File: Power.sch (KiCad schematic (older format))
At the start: 23 parts, among them U13 L78L12_SOT89, U14 MP4462, U3 L78L12_SOT89, U4 LP2985-3.3

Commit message: Lots of routing done
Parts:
- added C73: 1uF, Capacitor_SMD:C_0402_1005Metric, symbol Device:C_Small
- added C77: 10nF, Capacitor_SMD:C_0402_1005Metric, symbol Device:C_Small
- added C78: 2.2uF, Capacitor_SMD:C_0603_1608Metric, symbol Device:C_Small
- added U16: LP2985-3.3, Package_TO_SOT_SMD:SOT-23-5, symbol Regulator_Linear:LP2985-3.3
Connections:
- net labels added: +3V3_1, +3V3_2
- net labels removed: +3V3
- wire segments 51 -> 64
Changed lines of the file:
@@
 Connection ~ 8600 3600
-$Comp
-L power:+3V3 #PWR0123
-U 1 1 603A9DDE
-P 8600 3500
-F 0 "#PWR0123" H 8600 3350 50  0001 C CNN
-F 1 "+3V3" H 8615 3673 50  0000 C CNN
-F 2 "" H 8600 3500 50  0001 C CNN
-F 3 "" H 8600 3500 50  0001 C CNN
-	1    8600 3500
-	1    0    0    -1
-$EndComp
-Connection ~ 8600 3500
 $Comp
 L Device:C_Small C?
@@
 	7150 3050 7150 4050
 Wire Notes Line
-	7150 4050 8900 4050
-Wire Notes Line
-	8900 4050 8900 3050
-Wire Notes Line
-	8900 3050 7150 3050
+	10650 4050 10650 3050
 Text Notes 7200 3200 0    79   ~ 16
 3V3 LDO Regulator
@@
 	7050 4850 7050 4750
 Connection ~ 7050 4750
+$Comp
+L Regulator_Linear:LP2985-3.3 U16
+U 1 1 61219C4E
+P 9550 3600
+F 0 "U16" H 9550 3942 50  0000 C CNN
+F 1 "LP2985-3.3" H 9550 3851 50  0000 C CNN
+F 2 "Package_TO_SOT_SMD:SOT-23-5" H 9550 3925 50  0001 C CNN
+F 3 "http://www.ti.com/lit/ds/symlink/lp2985.pdf" H 9550 3600 50  0001 C CNN
+	1    9550 3600
+	1    0    0    -1
+$EndComp
+$Comp
+L Device:C_Small C?
+U 1 1 61219C54
+P 9050 3800
+AR Path="/61219C54" Ref="C?"  Part="1"
+AR Path="/60308500/61219C54" Ref="C73"  Part="1"
+F 0 "C73" H 9142 3846 50  0000 L CNN
+F 1 "1uF" H 9100 3800 50  0000 L CNN
+F 2 "Capacitor_SMD:C_0402_1005Metric" H 9050 3800 50  0001 C CNN
+F 3 "~" H 9050 3800 50  0001 C CNN
+	1    9050 3800
+	1    0    0    -1
+$EndComp
+$Comp
+L Device:C_Small C?
+U 1 1 61219C5A
+P 10050 3800
+AR Path="/61219C5A" Ref="C?"  Part="1"
+AR Path="/60308500/61219C5A" Ref="C77"  Part="1"
+F 0 "C77" H 10142 3846 50  0000 L CNN
+F 1 "10nF" H 10100 3800 50  0000 L CNN
+F 2 "Capacitor_SMD:C_0402_1005Metric" H 10050 3800 50  0001 C CNN
+F 3 "~" H 10050 3800 50  0001 C CNN
+	1    10050 3800
+	1    0    0    -1
+$EndComp
+Wire Wire Line
+	10050 3700 10050 3600
+Wire Wire Line
+	10050 3600 9950 3600
+Wire Wire Line
+	9050 3700 9050 3600
+Wire Wire Line
+	9050 3600 9150 3600
+Connection ~ 9050 3600
+Wire Wire Line
+	9050 3500 9150 3500
+$Comp
+L Device:C_Small C?
+U 1 1 61219C66
+P 10350 3800
+AR Path="/61219C66" Ref="C?"  Part="1"
+AR Path="/60308500/61219C66" Ref="C78"  Part="1"
+F 0 "C78" H 10442 3846 50  0000 L CNN
+F 1 "2.2uF" H 10400 3800 50  0000 L CNN
+F 2 "Capacitor_SMD:C_0603_1608Metric" H 10350 3800 50  0001 C CNN
+F 3 "~" H 10350 3800 50  0001 C CNN
+	1    10350 3800
+	1    0    0    -1
+$EndComp
+Wire Wire Line
+	10350 3700 10350 3600
+Wire Wire Line
+	10350 3600 10050 3600
+Connection ~ 10050 3600
+$Comp
+L power:GND #PWR?
+U 1 1 61219C6F
+P 9550 3900
+AR Path="/61219C6F" Ref="#PWR?"  Part="1"
+AR Path="/60308500/61219C6F" Ref="#PWR0113"  Part="1"
+F 0 "#PWR0113" H 9550 3650 50  0001 C CNN
+F 1 "GND" H 9650 3800 50  0000 C CNN
+F 2 "" H 9550 3900 50  0001 C CNN
+F 3 "" H 9550 3900 50  0001 C CNN
+	1    9550 3900
+	1    0    0    -1
+$EndComp
+Wire Wire Line
+	9050 3900 9550 3900
+Connection ~ 9550 3900
+Wire Wire Line
+	9550 3900 10050 3900
+Connection ~ 10050 3900
+Wire Wire Line
+	10050 3900 10350 3900
+Wire Wire Line
+	9950 3500 10350 3500
+Wire Wire Line
+	10350 3500 10350 3600
+Connection ~ 10350 3600
+Wire Wire Line
+	9050 3500 9050 3600
+$Comp
+L power:+5V #PWR0123
+U 1 1 61219C85
+P 9050 3500
+F 0 "#PWR0123" H 9050 3350 50  0001 C CNN
+F 1 "+5V" H 9065 3673 50  0000 C CNN
+F 2 "" H 9050 3500 50  0001 C CNN
+F 3 "" H 9050 3500 50  0001 C CNN
+	1    9050 3500
+	1    0    0    -1
+$EndComp
+Connection ~ 9050 3500
+Wire Notes Line
+	7150 3050 10650 3050
+Wire Notes Line
+	7150 4050 10650 4050
+$Comp
+L power:+3V3_1 #PWR0138
+U 1 1 612259E0
+P 8600 3500
+F 0 "#PWR0138" H 8600 3350 50  0001 C CNN
+F 1 "+3V3_1" H 8615 3673 50  0000 C CNN
+F 2 "" H 8600 3500 50  0001 C CNN
+F 3 "" H 8600 3500 50  0001 C CNN
+	1    8600 3500
+	1    0    0    -1
+$EndComp
+Connection ~ 8600 3500
+$Comp
+L power:+3V3_2 #PWR0145
+U 1 1 61226B90
+P 10350 3500
+F 0 "#PWR0145" H 10350 3350 50  0001 C CNN
+F 1 "+3V3_2" H 10365 3673 50  0000 C CNN
+F 2 "" H 10350 3500 50  0001 C CNN
+F 3 "" H 10350 3500 50  0001 C CNN
+	1    10350 3500
+	1    0    0    -1
+$EndComp
+Connection ~ 10350 3500
 $EndSCHEMATC

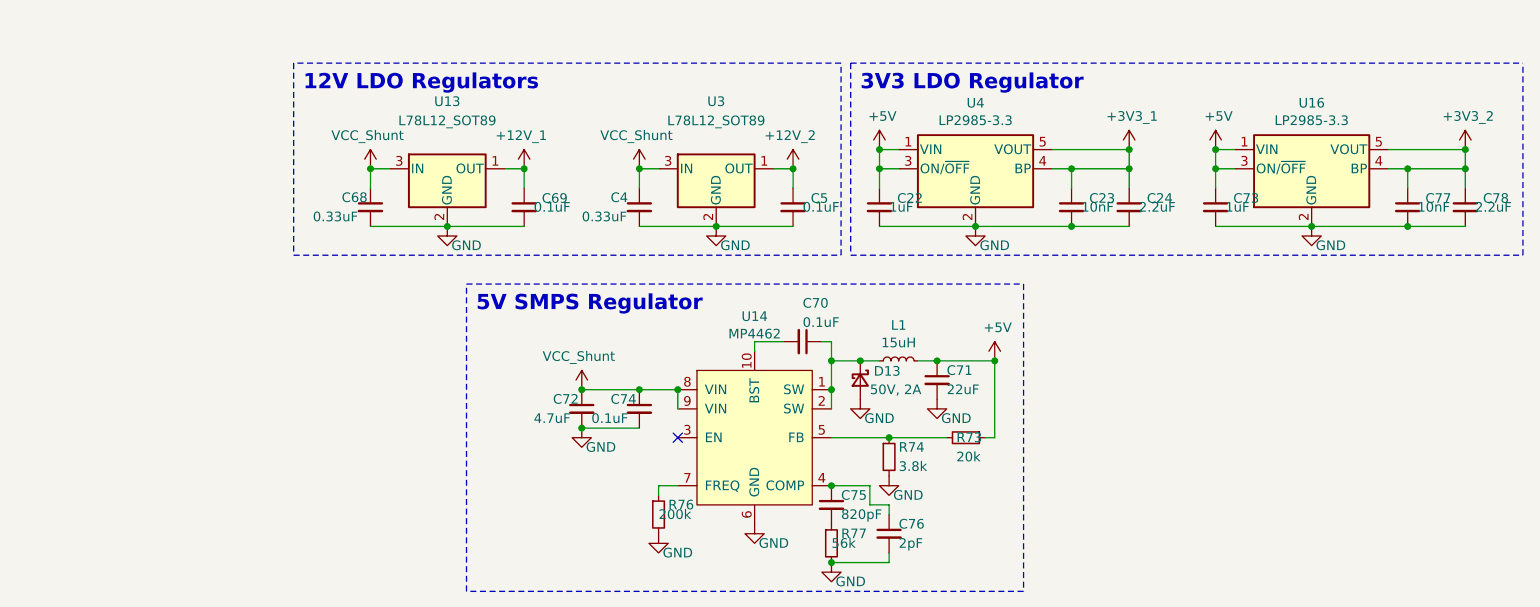
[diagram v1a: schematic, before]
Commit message: Added PNGs and PDFs
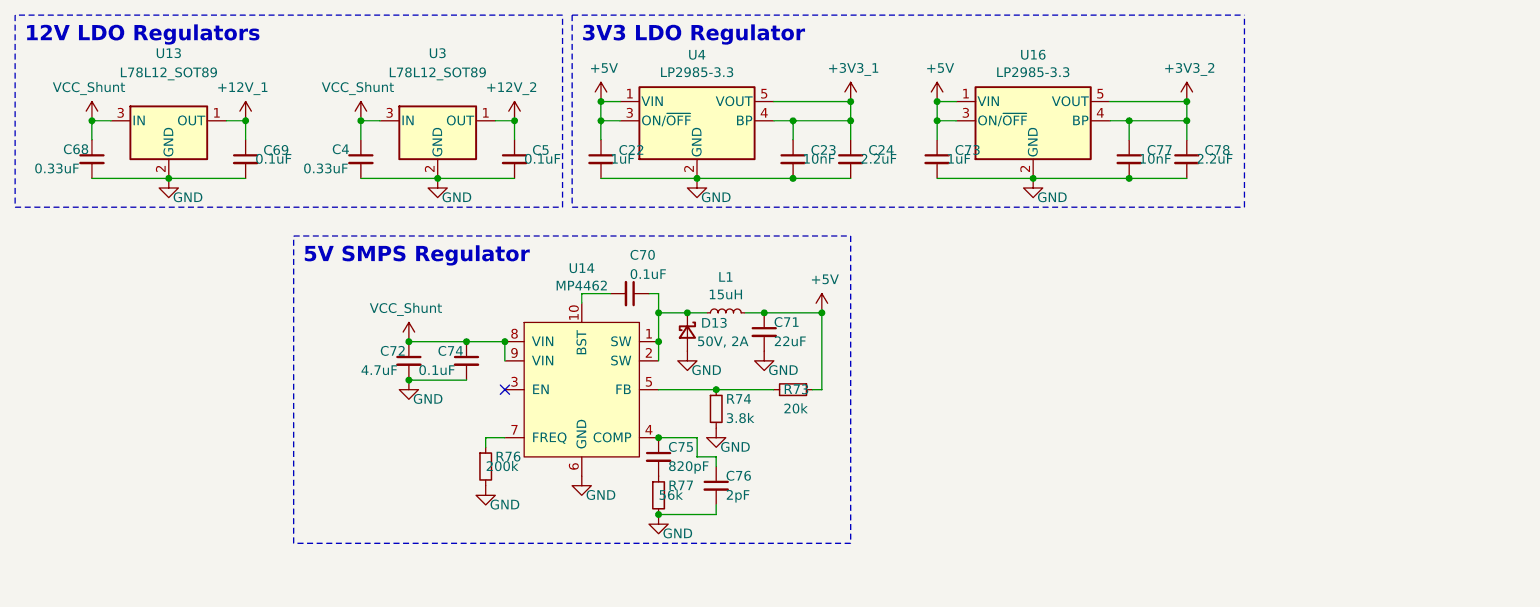
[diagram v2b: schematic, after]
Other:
- moved on the sheet: C22, C23, C24, C4, C5, C68, C69, C70, C71, C72, C73, C74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
